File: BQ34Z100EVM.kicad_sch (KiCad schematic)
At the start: 13 parts, among them IC1 BQ34Z100PWR-G1, J1 Conn_01x05_Pin, J2 Screw_Terminal_01x04, Q1 BSS138, Q2 BSS138

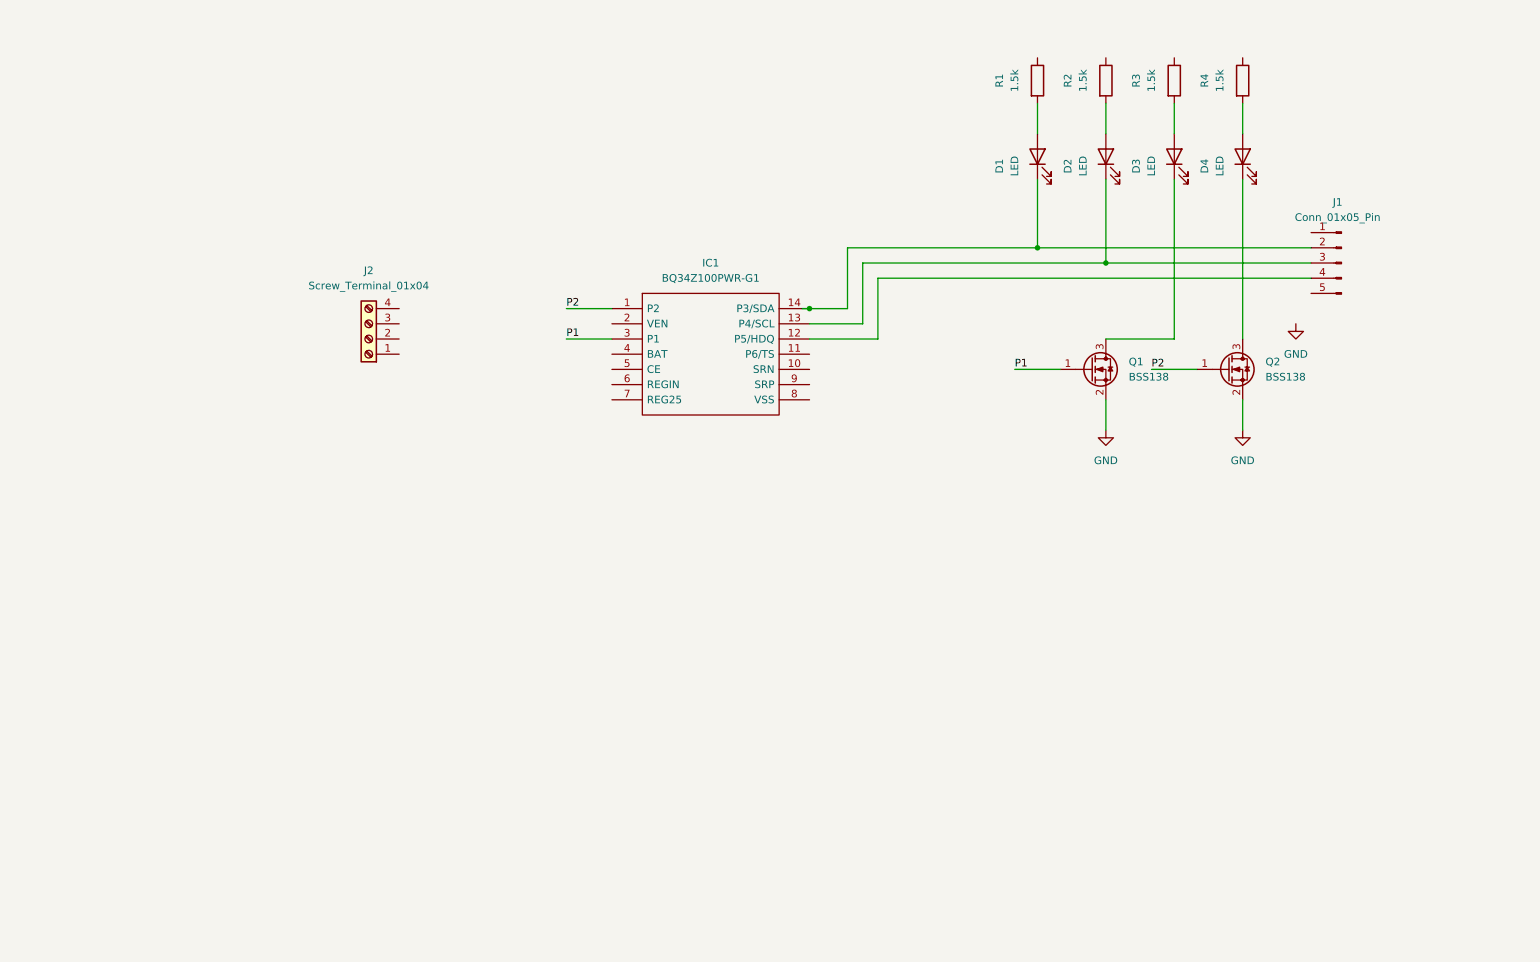
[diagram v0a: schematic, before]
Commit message: added schematic
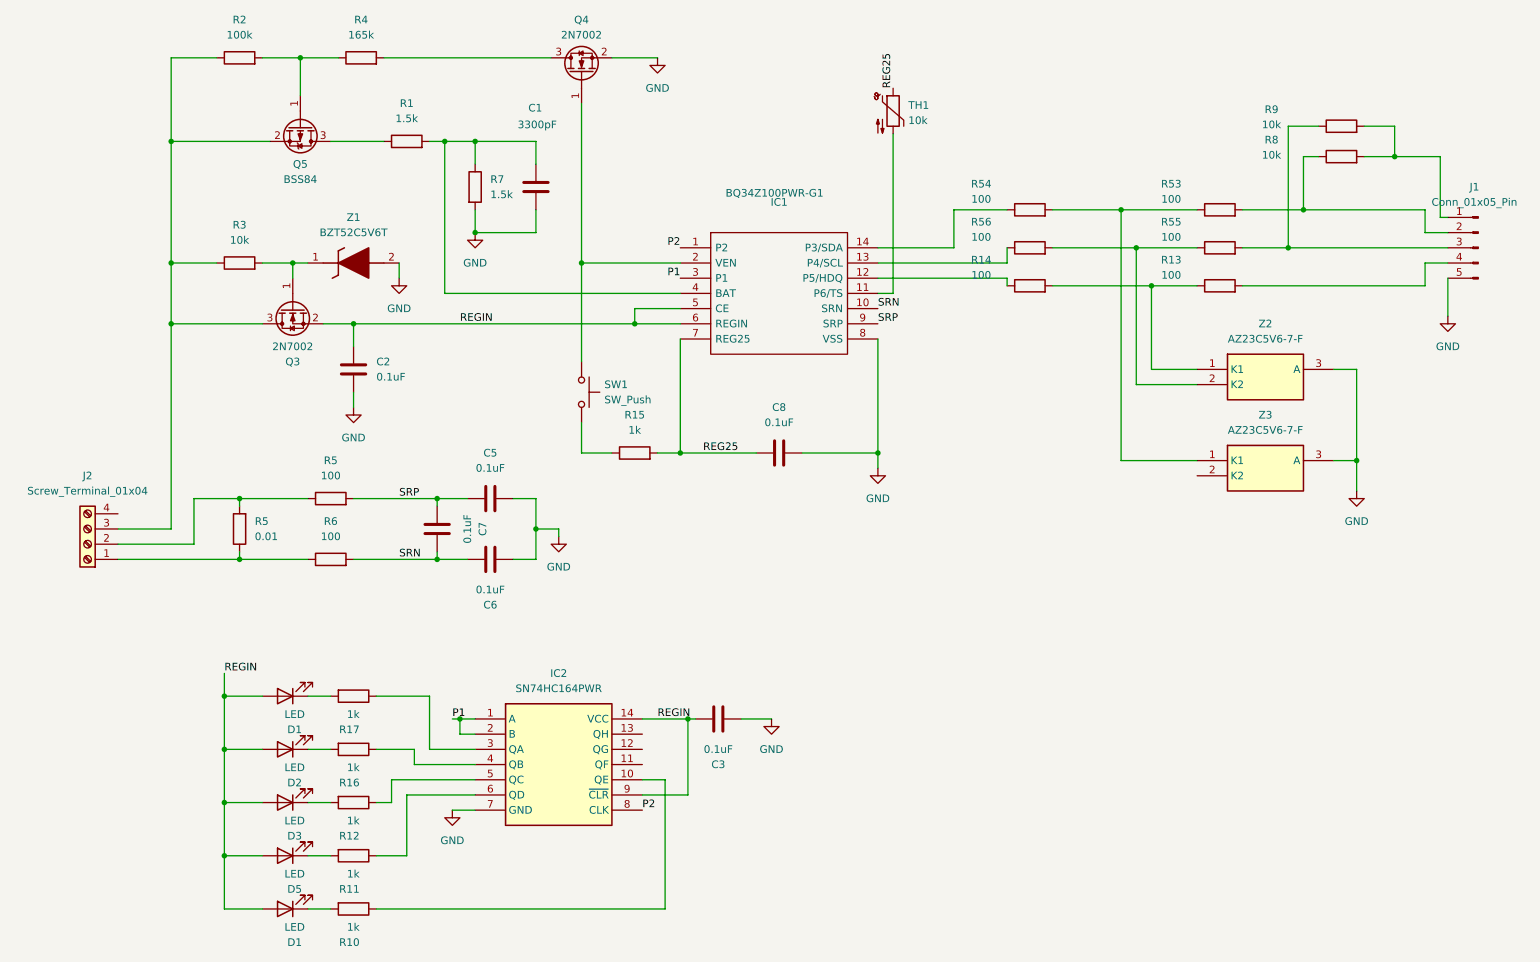
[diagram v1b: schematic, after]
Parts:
- removed D4: LED, symbol Device:LED
- removed Q1, Q2: BSS138, Package_TO_SOT_SMD:SOT-23, symbol Transistor_FET:BSS138
- added C1: 3300pF, symbol Device:C
- added C2, C3, C5, C6, C7, C8: 0.1uF, symbol Device:C
- added D1, D5: LED, symbol Device:LED
- added IC2: SN74HC164PWR, SOP65P640X120-14N, symbol SN74HC164PWR:SN74HC164PWR
- added Q3, Q4: 2N7002, Package_TO_SOT_SMD:SOT-23, symbol Transistor_FET:2N7002
- added Q5: BSS84, Package_TO_SOT_SMD:SOT-23, symbol Transistor_FET:BSS84
- added R10, R11, R12, R15, R16, R17: 1k, symbol Device:R
- added R13, R14, R5, R53, R54, R55, R56, R6: 100, symbol Device:R
- added R5: 0.01, symbol Device:R
- added R7: 1.5k, symbol Device:R
- added R8, R9: 10k, symbol Device:R
- added SW1: SW_Push, symbol Switch:SW_Push
- added TH1: 10k, symbol Device:Thermistor_NTC
- added Z1: BZT52C5V6T, SODFL1608X70N, symbol BZT52C5V6T:BZT52C5V6T
- added Z2, Z3: AZ23C5V6-7-F, SOT96P240X115-3N, symbol AZ23C5V6-7-F:AZ23C5V6-7-F
- R2: value 1.5k -> 100k
- R3: value 1.5k -> 10k
- R4: value 1.5k -> 165k
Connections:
- net GND: now also IC1.8 (VSS), J1.5 (Pin_5), C1.2, C2.2, C3.1, C5.2, C6.1, C8.2, IC2.7 (GND), Q4.2 (S), R7.2, Z1.2 (A), Z2.3 (A), Z3.3 (A)
- net P1: now also IC2.1 (A), IC2.2 (B)
- net P2: now also IC2.8 (CLK)
- net at R2.1: now also J2.3 (Pin_3), R3.1, Q3.3 (D), Q5.2 (S)
- net at R2.2: now also R4.1, Q5.1 (G); no longer D2.2 (A)
- net at D3.1 (K): now also R12.2
- net at J2.1 (Pin_1): now also R5.1, R6.1
- net at J2.2 (Pin_2): now also R5.1, R5.2
- net at R3.2: now also Q3.1 (G), Z1.1 (K); no longer D3.2 (A)
- net SRN: now reaches IC1.10 (SRN)
- net SRN: now also C6.2, C7.2, R6.2
- net at IC1.11 (P6/TS): now also TH1.2
- net at IC1.12 (P5/HDQ): now also R14.1; no longer J1.4 (Pin_4)
- net at IC1.2 (VEN): now also Q4.1 (G), SW1.1
- net at IC1.4 (BAT): no longer names the net of IC1.4 (BAT)
- net at IC1.4 (BAT): now also R1.2, C1.1, R7.1
- net REGIN: now reaches IC1.5 (CE)
- net REGIN: now also D1.2 (A), D2.2 (A), D3.2 (A), IC1.6 (REGIN), C2.1, C3.2, D1.2 (A), D5.2 (A), IC2.14 (VCC), IC2.9 (~{CLR}), Q3.2 (S)
- net REG25: now reaches IC1.7 (REG25)
- net REG25: now also C8.1, R15.2, TH1.1
- net SRP: now reaches IC1.9 (SRP)
- net SRP: now also C5.1, C7.1, R5.2
- net at R1.1: now also Q5.3 (D)
- net at J1.1 (Pin_1): now also R8.2, R9.2
- net at R4.2: now also Q4.3 (D)
- new net: J1.3 (Pin_3), R55.2, R9.1
- new net: IC1.13 (P4/SCL), R56.1
- new net: IC1.14 (P3/SDA), R54.1
- new net: R55.1, R56.2, Z2.2 (K2)
- new net: R53.1, R54.2, Z3.1 (K1)
- new net: R13.1, R14.2, Z2.1 (K1)
- new net: J1.4 (Pin_4), R13.2
- new net: D5.1 (K), R11.2
- new net: D2.1 (K), R16.2
- new net: IC2.10 (QE), R10.1
- new net: IC2.3 (QA), R17.1
- new net: IC2.4 (QB), R16.1
- new net: IC2.5 (QC), R12.1
- new net: IC2.6 (QD), R11.1
- new net: J1.2 (Pin_2), R53.2, R8.1
- new net: D1.1 (K), R10.2
- new net: D1.1 (K), R17.2
- new net: R15.1, SW1.2
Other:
- moved on the sheet: D1, IC1, J1, J2, R1, R3
